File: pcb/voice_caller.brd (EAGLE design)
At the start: 52.4 x 59.1 mm, 53 parts, among them IC1 PRO_MICRO, IC2 LM386M-1, IC3 78L12SMD, K1 TQ2SA-L2-5V, U1 25F32006WSOI

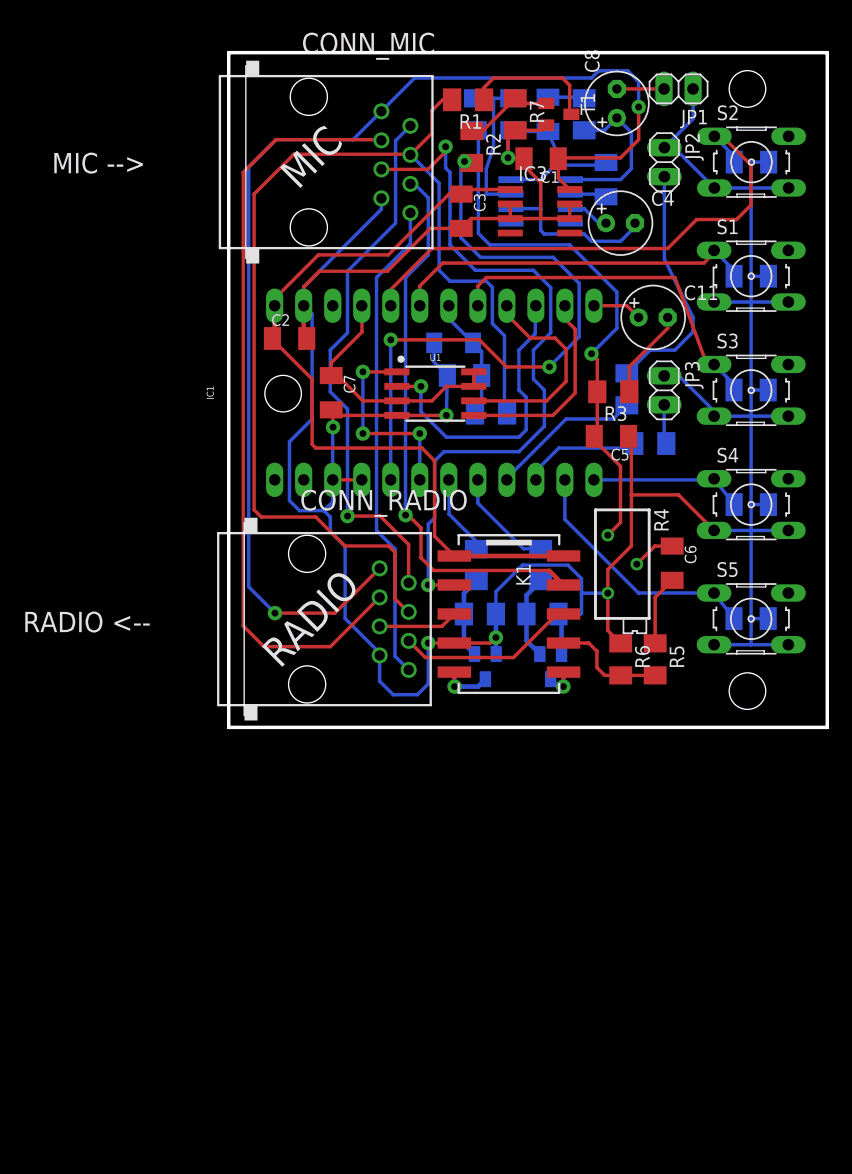
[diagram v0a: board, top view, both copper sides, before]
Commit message: Final adjustments.
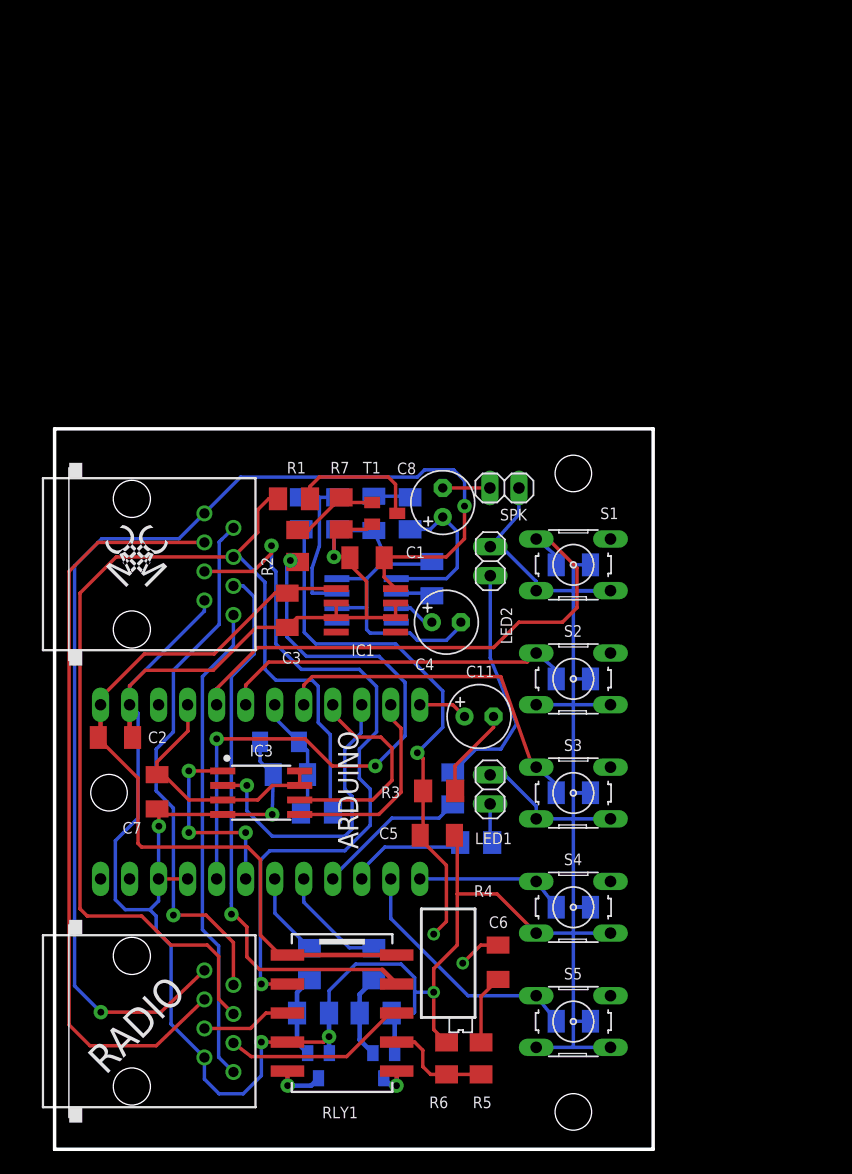
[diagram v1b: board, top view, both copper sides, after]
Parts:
- removed JP1, JP2, JP3: (no value), pinhead:1X02
- removed K1: TQ2SA-L2-5V, relay:TQ-SA
- removed U1: 25F32006WSOI, SparkFun-IC-Memory:SO08-EIAJ
- added ARDUINO: PRO_MICRO, SparkFun-Boards:SPARKFUN_PRO_MICRO
- added LED1, LED2, SPK: (no value), pinhead:1X02
- added RLY1: TQ2SA-L2-5V, relay:TQ-SA
- IC1: value PRO_MICRO -> 78L12SMD; device SparkFun-Boards:SPARKFUN_PRO_MICRO -> linear:SO08
- IC3: value 78L12SMD -> 25F32006WSOI; device linear:SO08 -> SparkFun-IC-Memory:SO08-EIAJ
- moved IC3 56.4 mm to (13.3, 0.00)
- moved S2 47.8 mm to (40.6, 9.96)
- moved C16 38.5 mm to (40.6, 19.9)
- moved C14 38.5 mm to (40.6, -10.0)
- moved C17 38.5 mm to (40.6, 9.96)
- moved S3 38.5 mm to (40.6, -0.03)
- moved S4 38.5 mm to (40.6, -10.0)
- moved S5 38.5 mm to (40.6, -20.0)
- moved C13 38.5 mm to (40.6, 0.00)
- moved C15 38.5 mm to (40.6, -20.0)
- moved CONN_MIC 38.4 mm to (2.00, 20.0)
- moved CONN_RADIO 38.4 mm to (2.00, -20.0)
- moved C10 38.1 mm to (28.3, 18.7)
- moved C11 38.1 mm to (32.4, 6.67)
- moved C12 38.1 mm to (15.9, 1.59)
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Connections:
- net +3V3: now also ARDUINO.21, IC3.3, IC3.7, IC3.8; no longer IC1.21, U1.3, U1.7, U1.8
- net +5V: now also ARDUINO.24, IC1.1, RLY1.1, RLY1.10; no longer IC1.24, IC3.1, K1.1, K1.10
- net +8V: now also IC1.8; no longer IC3.8
- net BUTTON1: now also ARDUINO.20, S1.1; no longer IC1.20, S2.1
- net BUTTON2: now also ARDUINO.19, S2.1; no longer IC1.19, S1.1
- net BUTTON3: now also ARDUINO.17; no longer IC1.17
- net BUTTON4: now also ARDUINO.12; no longer IC1.12
- net BUTTON5: now also ARDUINO.11; no longer IC1.11
- net FLASH_CS: now also ARDUINO.6, IC3.1; no longer IC1.6, U1.1
- net GND: now also ARDUINO.23, ARDUINO.3, ARDUINO.4, IC1.2, IC1.6, IC1.7, IC3.4, LED1.1, LED2.1, RLY1.4, SPK.1; no longer IC1.23, IC1.4, IC3.2, IC3.3, IC3.6, IC3.7, JP1.1, JP2.1, JP3.1, K1.4, U1.4
- net MIC: now also RLY1.9; no longer K1.9
- net MIC_GND: now also RLY1.2; no longer K1.2
- net MIC_GND_RADIO: now also RLY1.3; no longer K1.3
- net MIC_PWM: now also RLY1.7; no longer K1.7
- net MIC_RADIO: now also RLY1.8; no longer K1.8
- net MISO: now also ARDUINO.15, IC3.2; no longer IC1.15, U1.2
- net MOSI: now also ARDUINO.14, IC3.5; no longer IC1.14, U1.5
- net N$10: now also RLY1.5; no longer K1.5
- net N$12: now also ARDUINO.9; no longer IC1.9
- net N$13: now also RLY1.6; no longer K1.6
- net N$15: now also ARDUINO.10; no longer IC1.10
- net N$22: now also SPK.2; no longer JP1.2
- net N$4: now also LED2.2; no longer JP2.2
- net N$9: now also LED1.2; no longer JP3.2
- net PTT_SENSE: now also ARDUINO.18; no longer IC1.18
- net PTT_SW: now also ARDUINO.5; no longer IC1.5
- net PULSE_RX: now also ARDUINO.8; no longer IC1.8
- net PULSE_TX: now also ARDUINO.7; no longer IC1.7
- net PWM: now also ARDUINO.13; no longer IC1.13
- net SCK: now also ARDUINO.16, IC3.6; no longer IC1.16, U1.6
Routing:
- net GND: track 330.9 -> 335.8 mm
- net BUTTON3: track 31.0 -> 31.9 mm
- net BUTTON1: track 46.8 -> 47.7 mm
- net MIC_GND_RADIO: track 6.98 -> 7.83 mm
- net MIC: track 48.6 -> 49.3 mm
- net MIC_GND: track 63.2 -> 63.9 mm
- net AF_OUT: track 67.5 -> 66.8 mm
- net +5V: track 69.1 -> 69.8 mm
- net PULSE_RX: track 9.20 -> 9.84 mm
- net MIC_PWM: track 10.0 -> 9.39 mm
- net MIC_RADIO: track 15.7 -> 16.3 mm
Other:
- board size 52.4 x 59.1 mm -> 52.4 x 63.1 mm
- board text removed: "MIC -->"
- board text removed: "RADIO <--"
